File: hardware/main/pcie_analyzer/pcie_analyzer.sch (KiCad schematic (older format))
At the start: 51 parts, among them J1 HDR40, J2 HDR40, J3 Conn_Coaxial, J4 Conn_Coaxial, J5 Conn_Coaxial, J6 Conn_Coaxial, J7 Conn_Coaxial, J8 Conn_Coaxial

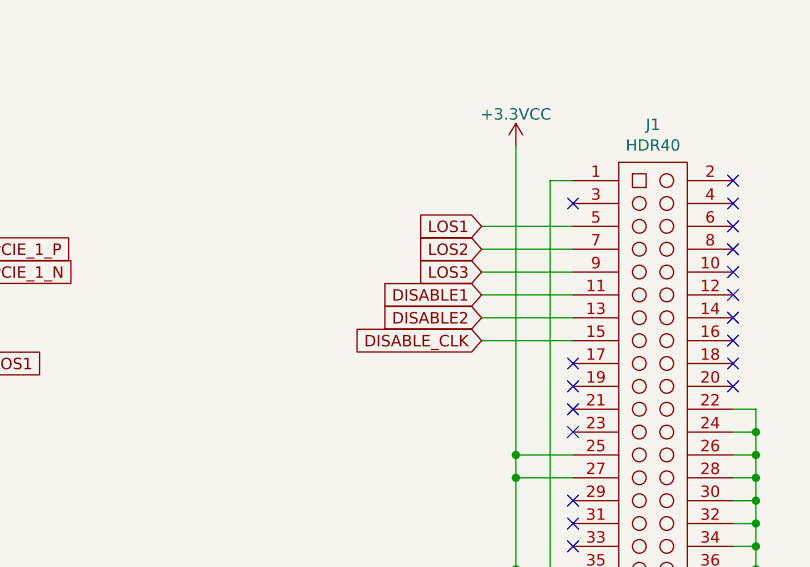
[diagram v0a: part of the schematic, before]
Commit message: pcb work
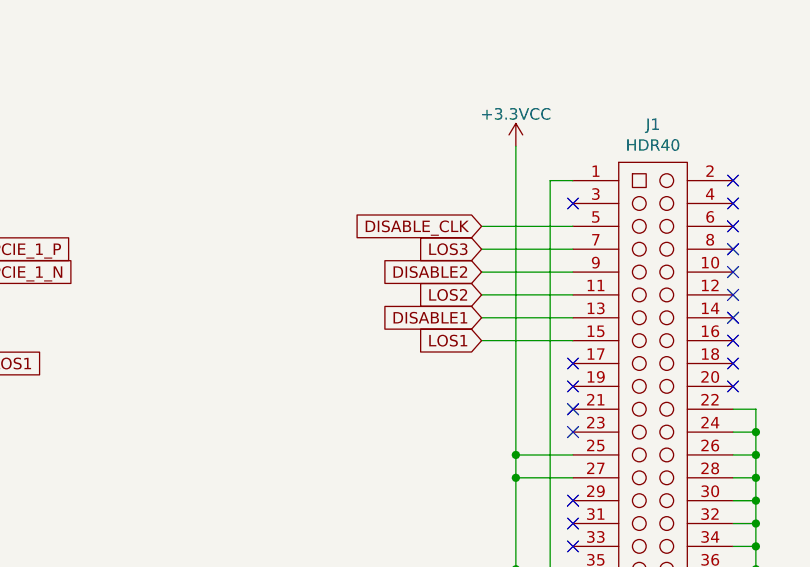
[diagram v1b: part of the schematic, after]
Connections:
- net DISABLE1: now also J1.13; no longer J1.11
- net DISABLE2: now also J1.9; no longer J1.13
- net DISABLE_CLK: now also J1.5; no longer J1.15
- net LOS1: now also J1.15; no longer J1.5
- net LOS2: now also J1.11; no longer J1.7
- net LOS3: now also J1.7; no longer J1.9
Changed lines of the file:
@@
 Wire Wire Line
 	2300 2500 2700 2500
-Text GLabel 11800 2000 0    50   Input ~ 0
+Text GLabel 11800 2500 0    50   Input ~ 0
 LOS1
-Text GLabel 11800 2100 0    50   Input ~ 0
+Text GLabel 11800 2300 0    50   Input ~ 0
 LOS2
+Text GLabel 11800 2400 0    50   Input ~ 0
+DISABLE1
 Text GLabel 11800 2200 0    50   Input ~ 0
-LOS3
-Text GLabel 11800 2300 0    50   Input ~ 0
-DISABLE1
-Text GLabel 11800 2400 0    50   Input ~ 0
 DISABLE2
-Text GLabel 11800 2500 0    50   Input ~ 0
-DISABLE_CLK
 Wire Wire Line
 	11800 2000 12200 2000
@@
 NoConn ~ 14400 1900
 NoConn ~ 14400 2000
+Text GLabel 11800 2000 0    50   Input ~ 0
+DISABLE_CLK
+Text GLabel 11800 2100 0    50   Input ~ 0
+LOS3
 $EndSCHEMATC

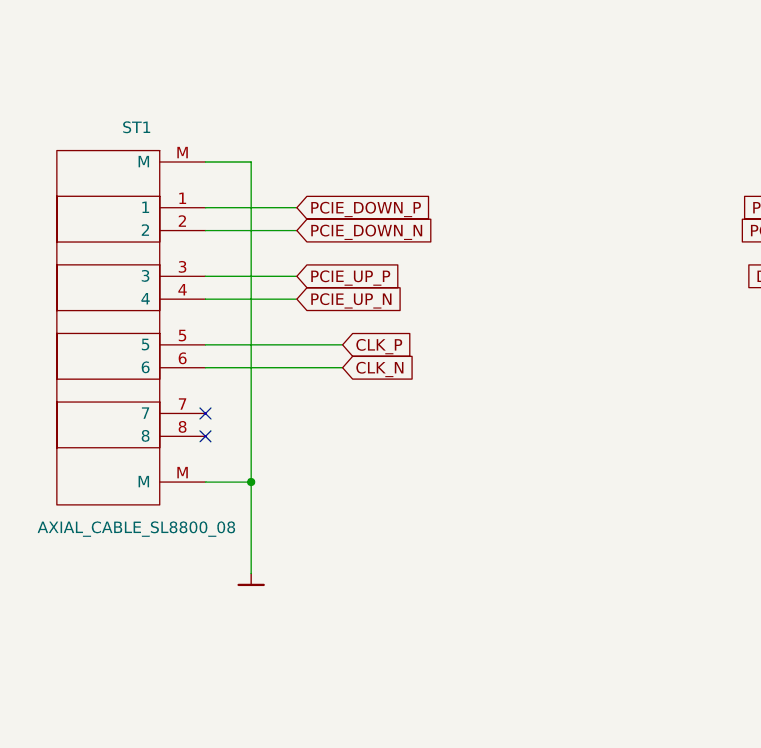
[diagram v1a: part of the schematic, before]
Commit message: first release sch/pcb
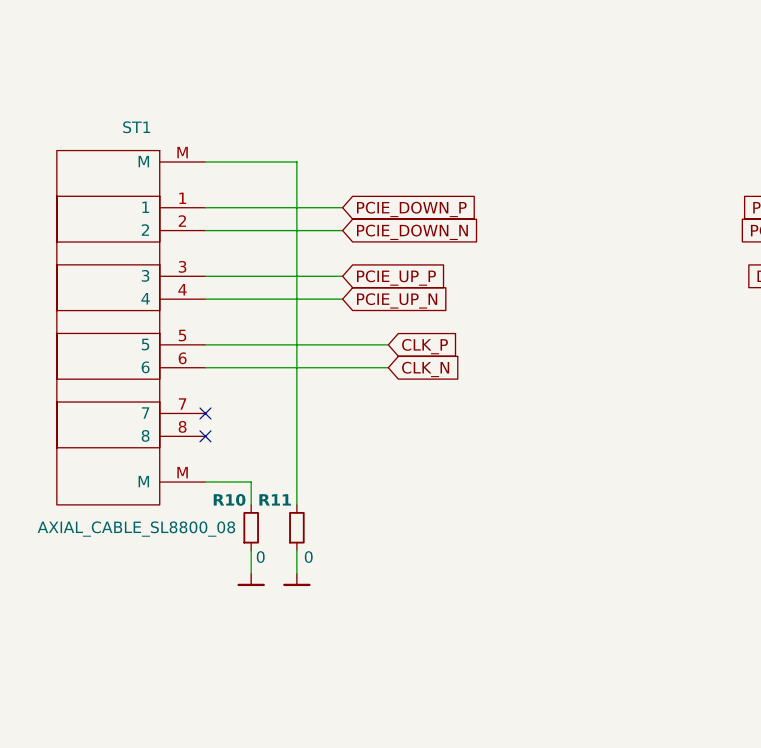
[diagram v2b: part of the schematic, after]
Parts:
- added R10, R11: 0, ecp5_pcie_analyzer:R_0402, symbol pcie_analyzer:R
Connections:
- net GND: now also R10.2, R11.2; no longer ST1.M
- new net: R10.1, ST1.M
- new net: R11.1, ST1.M
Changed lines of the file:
@@
 	2300 3300 2500 3300
 Wire Wire Line
-	2500 3300 2500 3700
-Wire Wire Line
-	2300 1900 2500 1900
-Wire Wire Line
-	2500 1900 2500 3300
-Connection ~ 2500 3300
-Text GLabel 2700 2400 2    50   Input ~ 0
+	2500 3300 2500 3400
+Text GLabel 2900 2400 2    50   Input ~ 0
 PCIE_UP_P
-Text GLabel 2900 2700 2    50   Input ~ 0
+Text GLabel 3100 2700 2    50   Input ~ 0
 CLK_P
-Text GLabel 2900 2800 2    50   Input ~ 0
+Text GLabel 3100 2800 2    50   Input ~ 0
 CLK_N
-Wire Wire Line
-	2300 2100 2700 2100
-Wire Wire Line
-	2300 2200 2700 2200
-Wire Wire Line
-	2300 2400 2700 2400
-Wire Wire Line
-	2300 2700 2900 2700
-Wire Wire Line
-	2300 2800 2900 2800
 NoConn ~ 2300 3000
 NoConn ~ 2300 3100
@@
 Wire Wire Line
 	5100 5600 6200 5600
-Text GLabel 2700 2200 2    50   Input ~ 0
+Text GLabel 2900 2200 2    50   Input ~ 0
 PCIE_DOWN_N
-Text GLabel 2700 2100 2    50   Input ~ 0
+Text GLabel 2900 2100 2    50   Input ~ 0
 PCIE_DOWN_P
 Wire Wire Line
@@
 	0    1    1    0
 $EndComp
-Text GLabel 2700 2500 2    50   Input ~ 0
+Text GLabel 2900 2500 2    50   Input ~ 0
 PCIE_UP_N
-Wire Wire Line
-	2300 2500 2700 2500
 Text GLabel 11800 2500 0    50   Input ~ 0
 LOS1
@@
 Text GLabel 11800 2100 0    50   Input ~ 0
 LOS3
+Wire Wire Line
+	2500 3600 2500 3700
+$Comp
+L pcie_analyzer:R R11
+U 1 1 6125E84F
+P 2700 3500
+F 0 "R11" H 2530 3620 50  0000 L CNB
+F 1 "0" H 2730 3370 50  0000 L CNN
+F 2 "ecp5_pcie_analyzer:R_0402" V 2630 3500 50  0001 C CNN
+F 3 "" H 2700 3500 50  0001 C CNN
+	1    2700 3500
+	1    0    0    -1
+$EndComp
+$Comp
+L pcie_analyzer:GND #PWR0127
+U 1 1 61278318
+P 2700 3700
+F 0 "#PWR0127" H 2695 3530 50  0001 C CNN
+F 1 "GND" H 2700 3600 50  0001 C CNN
+F 2 "" H 2700 3700 50  0001 C CNN
+F 3 "" H 2700 3700 50  0001 C CNN
+	1    2700 3700
+	1    0    0    -1
+$EndComp
+Wire Wire Line
+	2700 3600 2700 3700
+$Comp
+L pcie_analyzer:R R10
+U 1 1 6125D88C
+P 2500 3500
+F 0 "R10" H 2330 3620 50  0000 L CNB
+F 1 "0" H 2520 3370 50  0000 L CNN
+F 2 "ecp5_pcie_analyzer:R_0402" V 2430 3500 50  0001 C CNN
+F 3 "" H 2500 3500 50  0001 C CNN
+	1    2500 3500
+	1    0    0    -1
+$EndComp
+Wire Wire Line
+	2300 2100 2900 2100
+Wire Wire Line
+	2300 2200 2900 2200
+Wire Wire Line
+	2300 2400 2900 2400
+Wire Wire Line
+	2300 2500 2900 2500
+Wire Wire Line
+	2300 2700 3100 2700
+Wire Wire Line
+	2300 2800 3100 2800
+Wire Wire Line
+	2700 1900 2700 3400
+Wire Wire Line
+	2300 1900 2700 1900
 $EndSCHEMATC

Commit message: major design update
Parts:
- ST1: symbol pcie_analyzer:AXIAL_CABLE_SL8800_08 -> pcie_analyzer-rescue:AXIAL_CABLE_SL8800_08-pcie_analyzer
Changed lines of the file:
@@
 	13600 8600 13600 8700
 $Comp
-L pcie_analyzer:AXIAL_CABLE_SL8800_08 ST1
+L pcie_analyzer-rescue:AXIAL_CABLE_SL8800_08-pcie_analyzer ST1
 U 1 1 611C5899
 P 2300 1900
